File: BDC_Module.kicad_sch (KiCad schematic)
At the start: 28 parts, among them J1 Conn_01x10_Pin, J2 Conn_01x10_Pin, J3 Conn_01x10_Pin, J4 Conn_01x02, J5 Conn_01x02, U1 TPS54531DDA

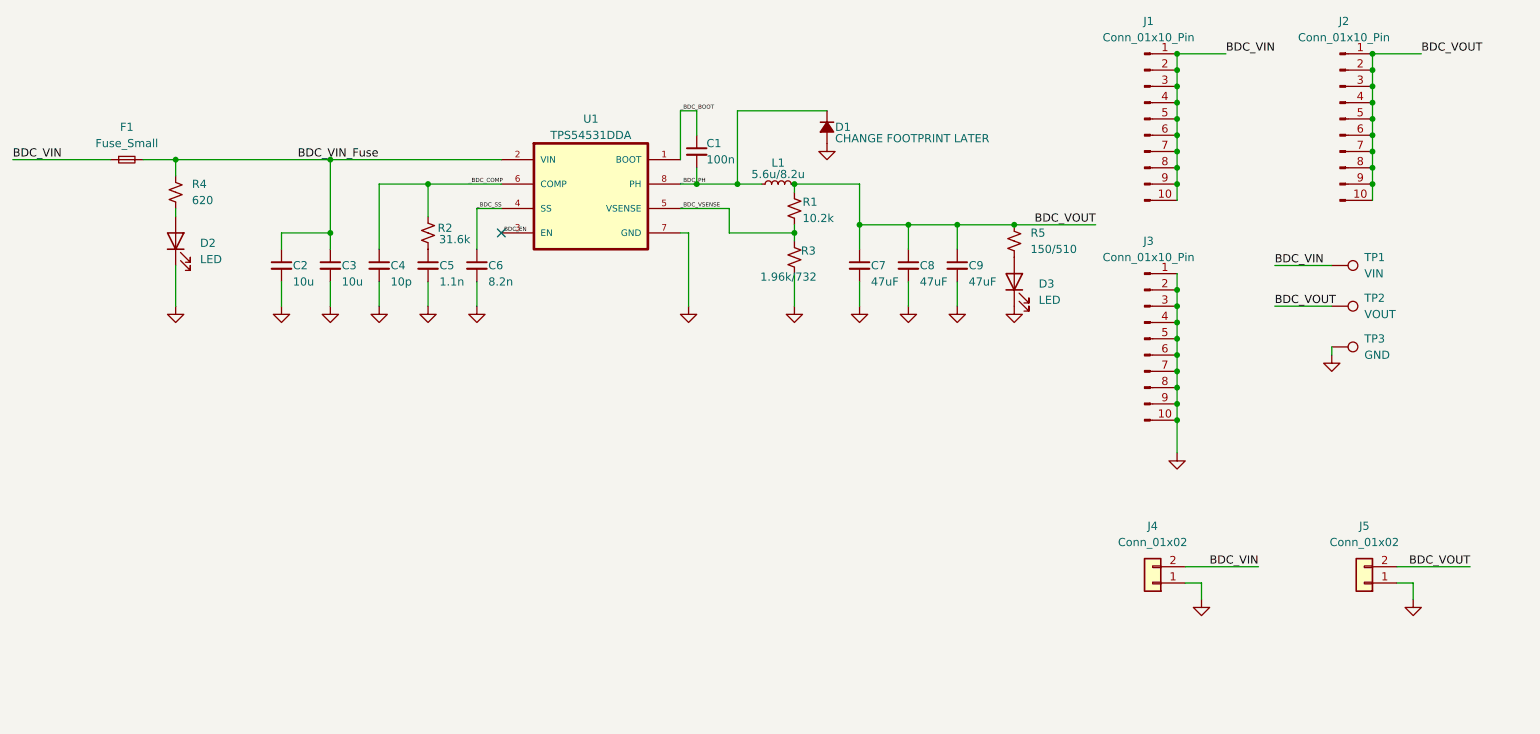
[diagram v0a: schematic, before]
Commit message: update mounting
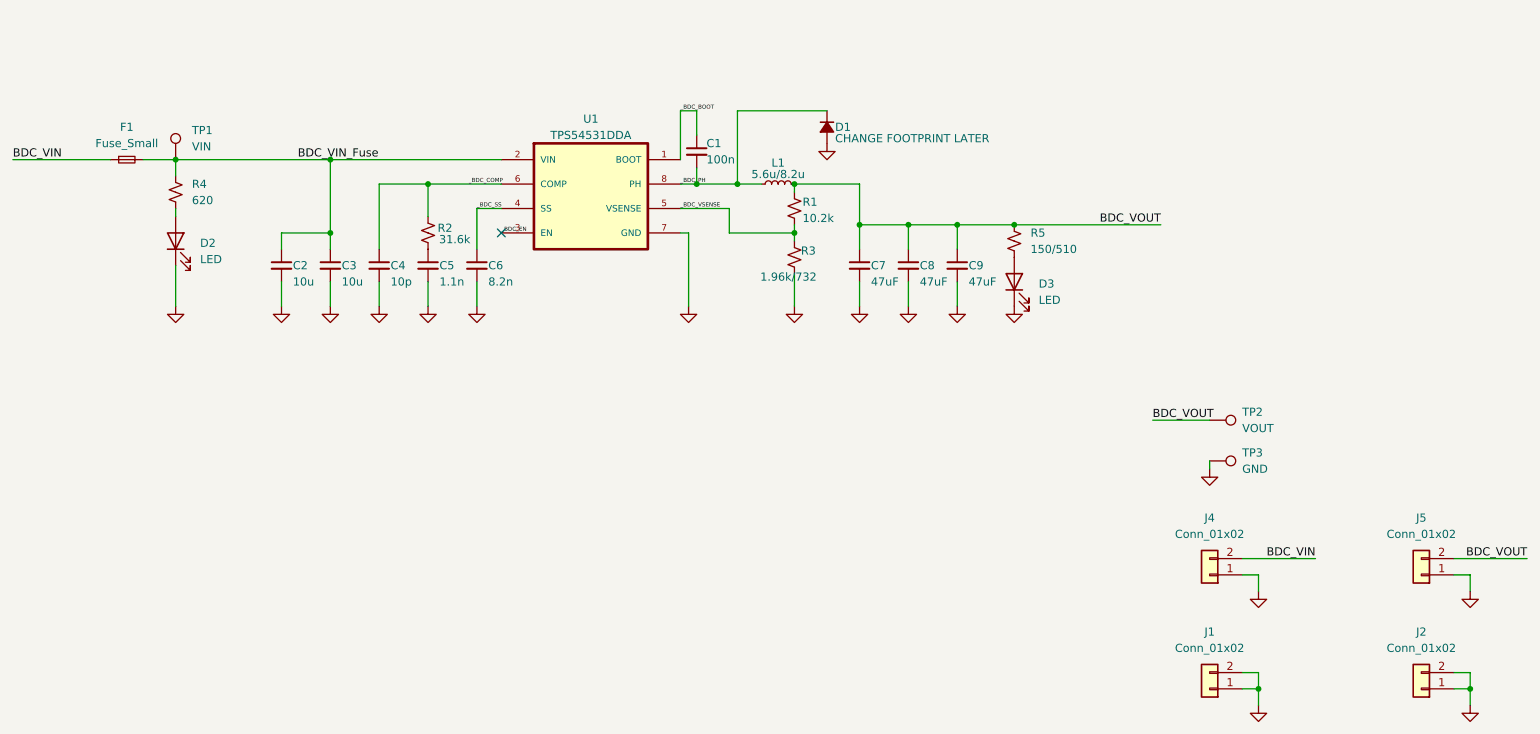
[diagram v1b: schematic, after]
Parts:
- removed J1, J2, J3: Conn_01x10_Pin, Connector_PinHeader_2.54mm:PinHeader_1x10_P2.54mm_Vertical, symbol Connector:Conn_01x10_Pin
- added J1, J2: Conn_01x02, Connector_AMASS:AMASS_XT30U-F_1x02_P5.0mm_Vertical, symbol Connector_Generic:Conn_01x02
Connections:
- net BDC_VIN: no longer TP1.1
- net BDC_VIN_Fuse: now also TP1.1
- net GND: now also J1.1 (Pin_1), J1.2 (Pin_2), J2.1 (Pin_1), J2.2 (Pin_2)
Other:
- moved on the sheet: J4, J5, TP1, TP2, TP3
